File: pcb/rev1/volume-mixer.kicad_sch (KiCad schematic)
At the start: 144 parts, among them CON1 TC2030-IDC, J1 Conn_01x04_Pin, J10 Conn_01x04_Pin, J2 Conn_01x10_Pin, J3 Conn_01x04_Pin, J4 Conn_01x10_Pin, J5 JST, J6 Conn_01x04_Pin, J7 Conn_01x04_Pin, J8 Conn_01x04_Pin, J9 Conn_01x04_Pin, Q1 NMOS, Q2 NMOS, Q3 NMOS, Q4 NMOS, Q5 NMOS, Q6 NMOS, Q7 NMOS, Q8 NMOS, Q9 NMOS, SW2 SW_Push, U1 STM32F302C8Tx, U2 24LC64, U3 XC6206PxxxMR, U4 XC6206PxxxMR, U5 PRTR5V0U2X, U6 TCA9548APWR, Y1 8MHz

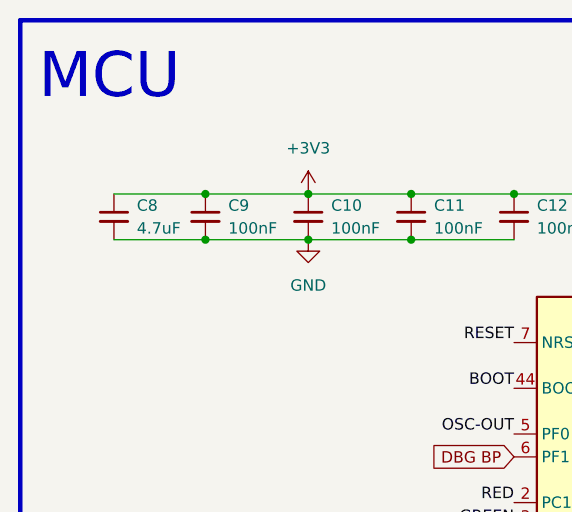
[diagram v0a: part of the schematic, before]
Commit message: V1
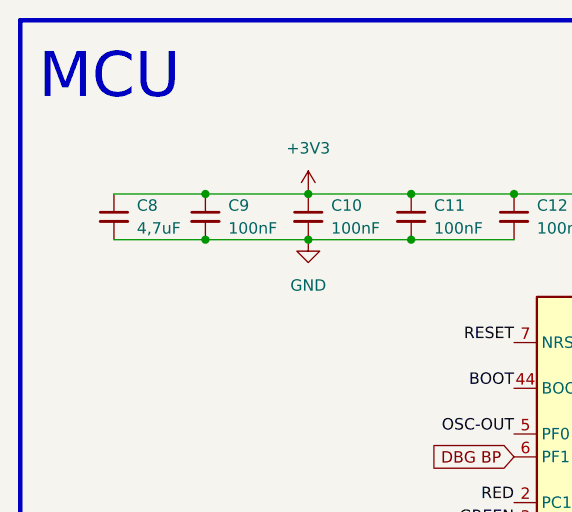
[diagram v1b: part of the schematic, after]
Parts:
- C18, C24: footprint Capacitor_SMD:C_0603_1608Metric -> Capacitor_SMD:C_0805_2012Metric
- C8: value 4.7uF -> 4,7uF
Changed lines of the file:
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@@
 			)
 		)
-		(property "Footprint" "Capacitor_SMD:C_0603_1608Metric"
+		(property "Footprint" "Capacitor_SMD:C_0805_2012Metric"
 			(at 34.29 115.57 0)
 			(effects
@@
 			)
 		)
-		(property "Value" "4.7uF"
+		(property "Value" "4,7uF"
 			(at 25.4 35.5662 0)
 			(effects
@@
 			)
 		)
-		(property "Footprint" "Capacitor_SMD:C_0603_1608Metric"
+		(property "Footprint" "Capacitor_SMD:C_0805_2012Metric"
 			(at 34.29 95.25 0)
 			(effects
